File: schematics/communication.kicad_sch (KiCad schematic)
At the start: 9 parts, among them J2 Conn_01x05_Pin, U3 SHT31-DIS

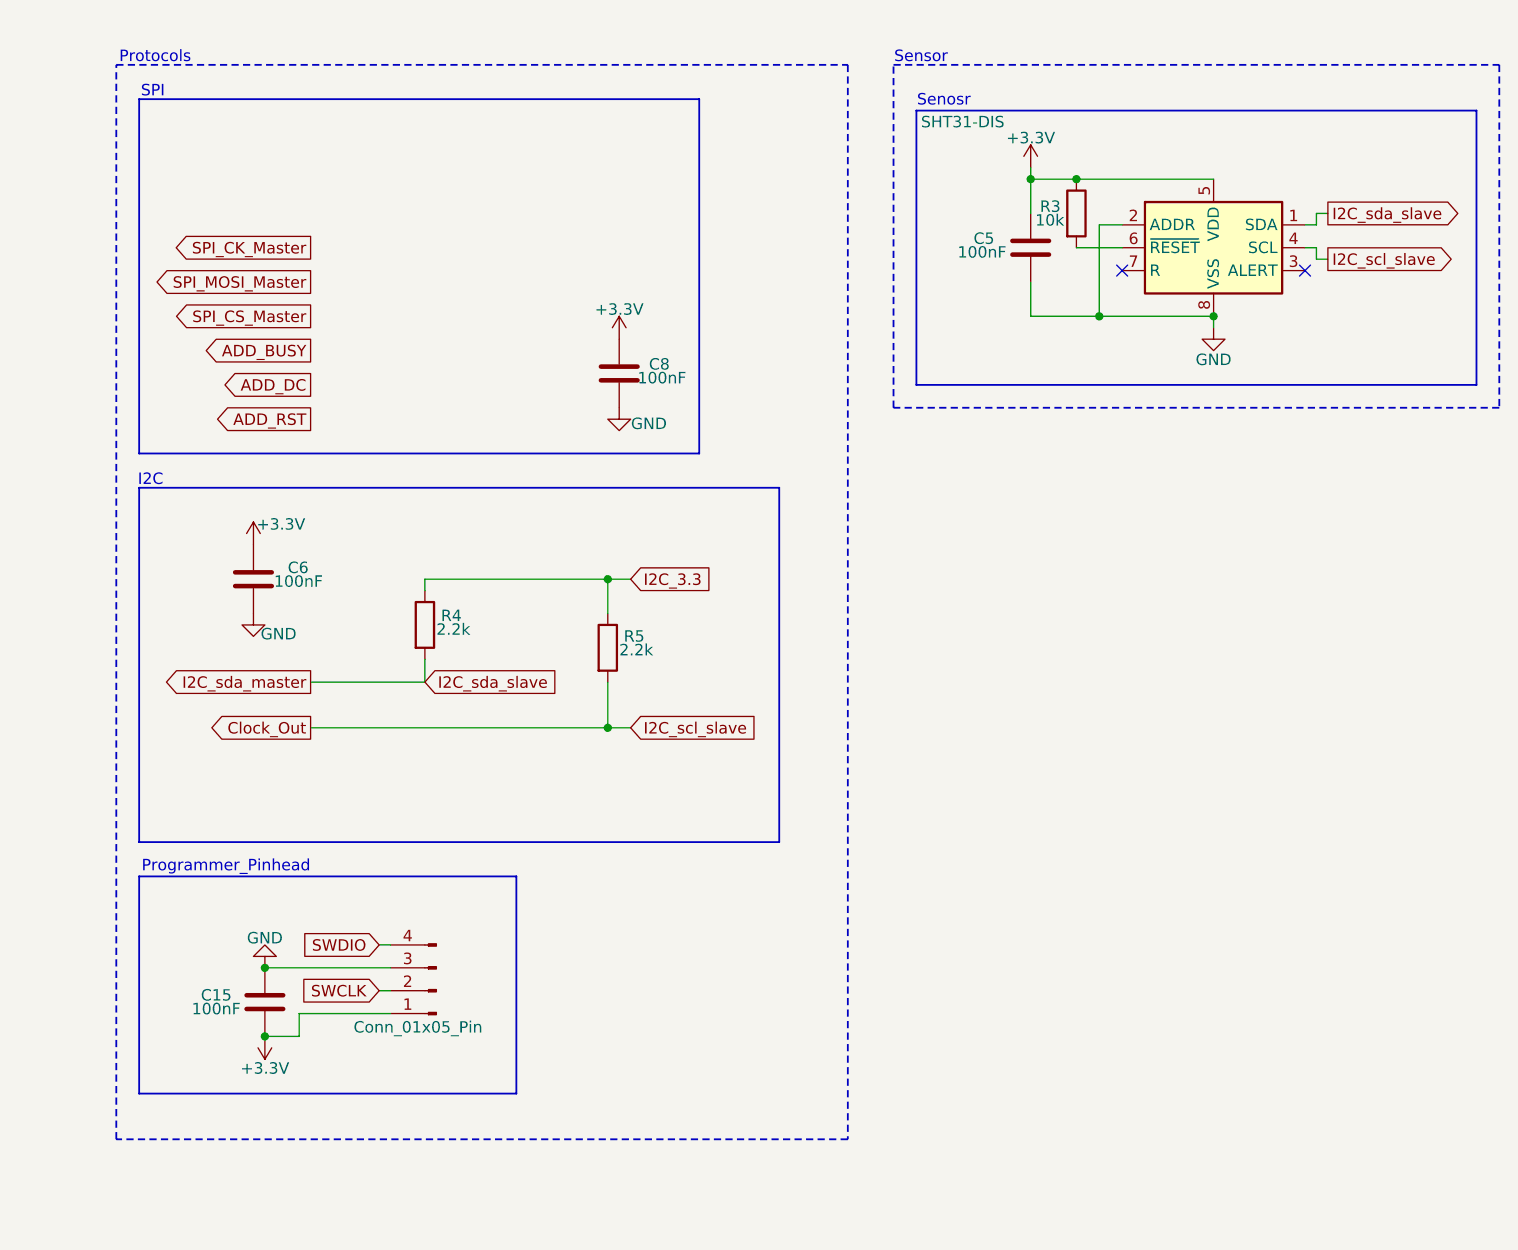
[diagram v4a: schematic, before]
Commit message: 2026-03-01 | 2
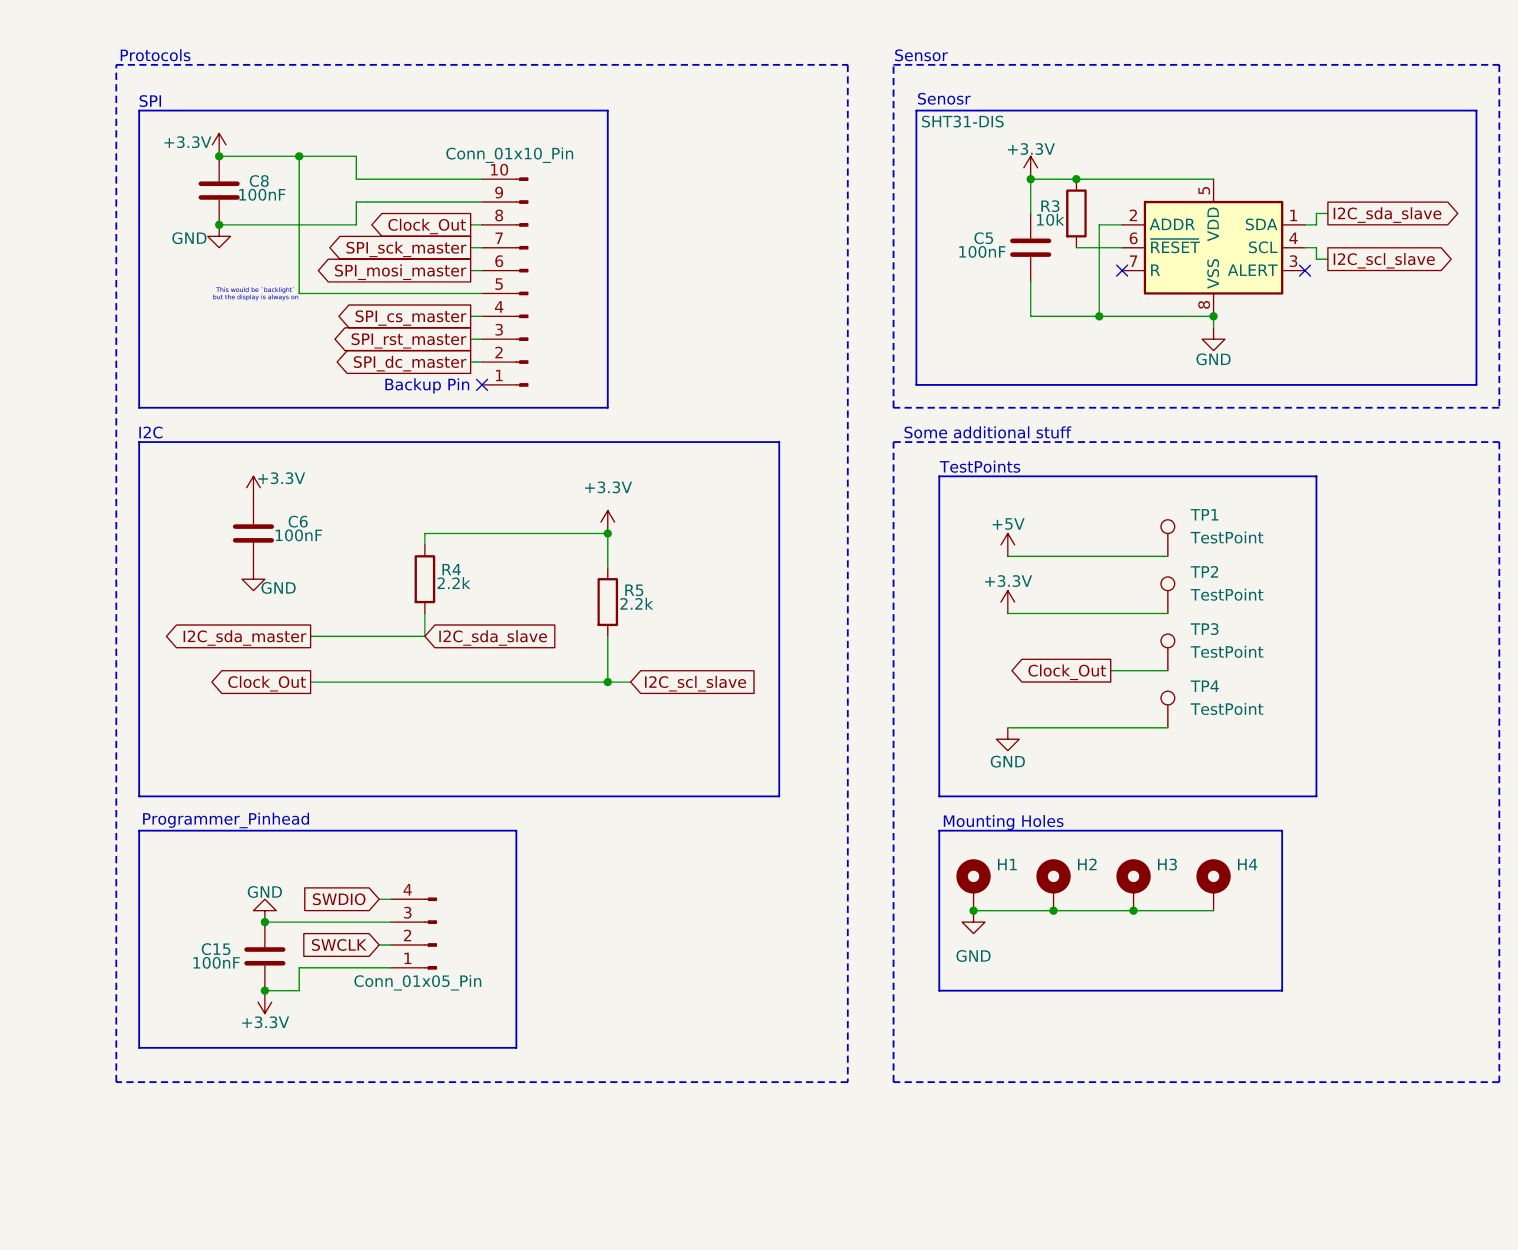
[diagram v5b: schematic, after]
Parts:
- added H1, H2, H3, H4: MountingHole_Pad, MountingHole:MountingHole_2.2mm_M2_DIN965_Pad, symbol Mechanical:MountingHole_Pad
- added J3: Conn_01x10_Pin, Connector_PinHeader_1.00mm:PinHeader_1x10_P1.00mm_Vertical, symbol Connector:Conn_01x10_Pin
- added TP1, TP2, TP3, TP4: TestPoint, TestPoint:TestPoint_Pad_1.0x1.0mm, symbol Connector:TestPoint
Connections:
- net I2C_3.3 is gone; now on net +3.3V: R4.1, R5.1
- net +3.3V: now also J3.10 (Pin_10), J3.5 (Pin_5), TP2.1
- net Clock_Out: now also J3.8 (Pin_8), TP3.1
- net GND: now also H1.1, H2.1, H3.1, H4.1, J3.9 (Pin_9), TP4.1
- new net +5V: TP1.1
- new net SPI_cs_master: J3.4 (Pin_4)
- new net SPI_dc_master: J3.2 (Pin_2)
- new net SPI_mosi_master: J3.6 (Pin_6)
- new net SPI_rst_master: J3.3 (Pin_3)
- new net SPI_sck_master: J3.7 (Pin_7)
- no-connect marks 2 -> 3
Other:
- note added: "Backup Pin"
- note added: "Mounting Holes"
- note added: "Some additional stuff"
- note added: "TestPoints"
- note added: "This would be `backlight` but the display is always on"
- moved on the sheet: C15, C6, C8, R4, R5

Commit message: 2026-03-09 | So-Mo
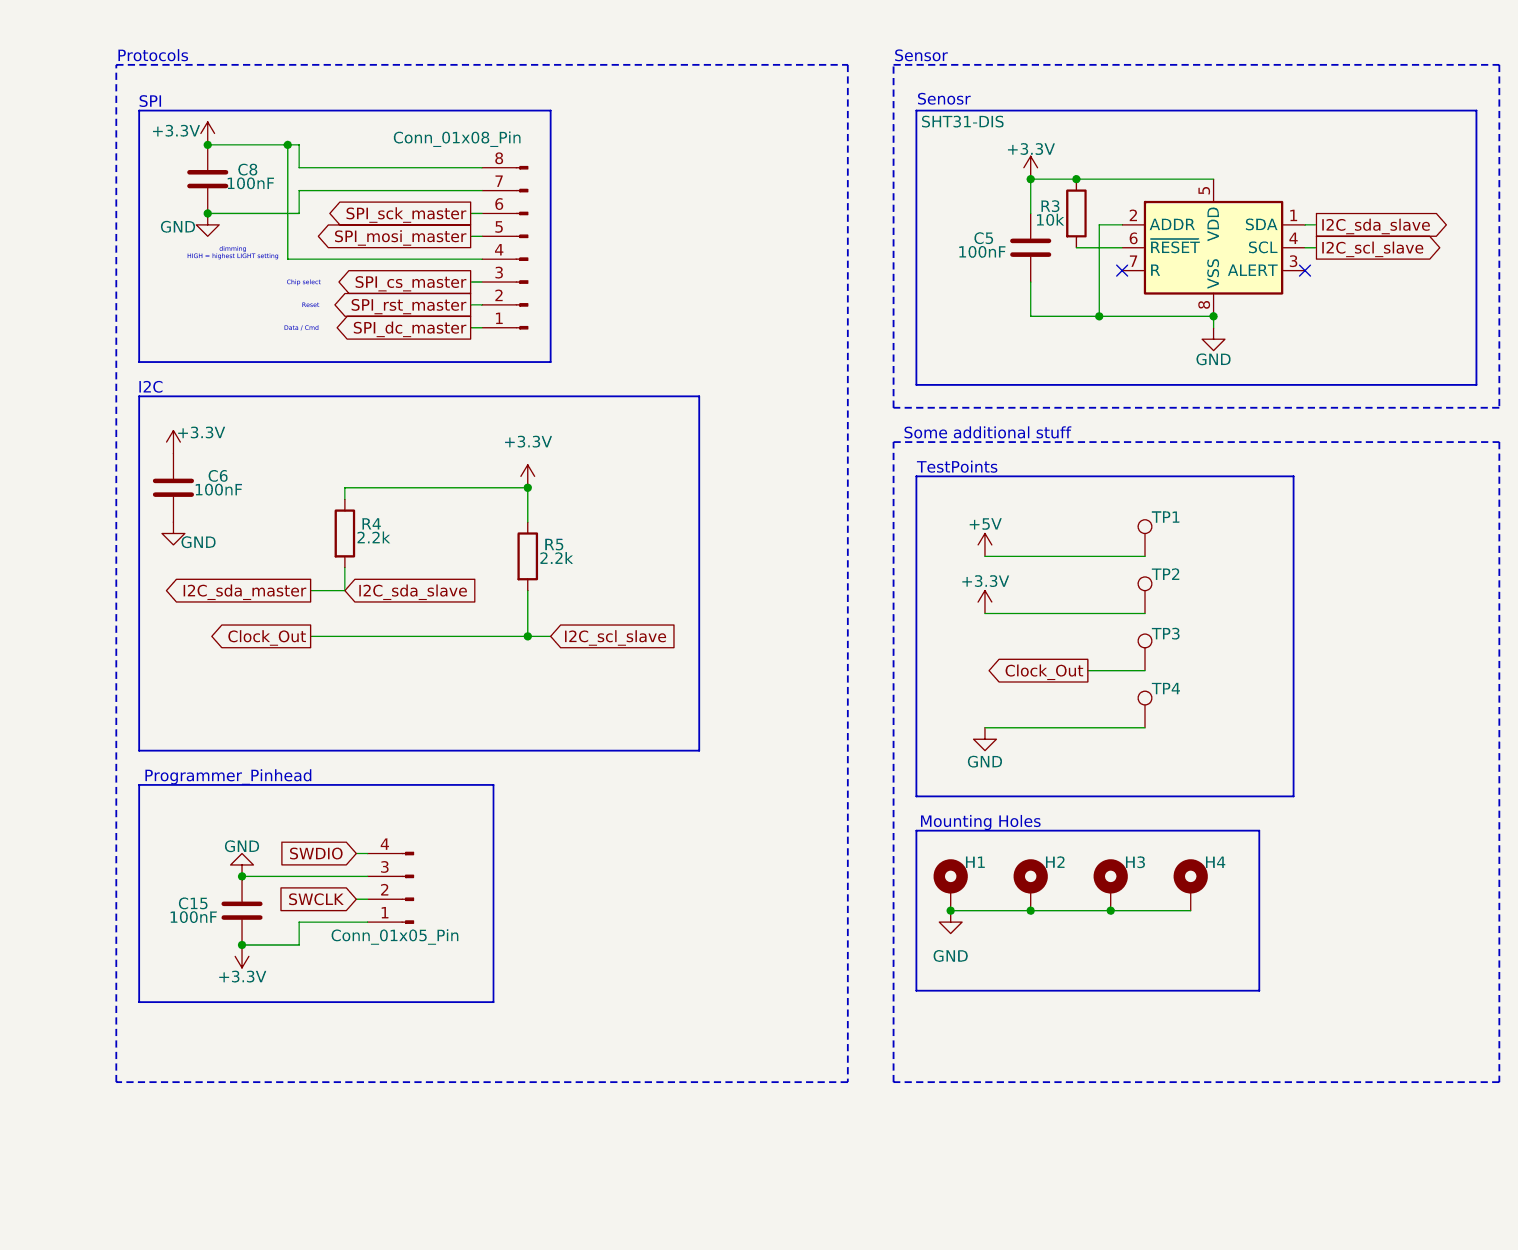
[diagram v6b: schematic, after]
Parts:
- removed J3: Conn_01x10_Pin, Connector_PinHeader_1.00mm:PinHeader_1x10_P1.00mm_Vertical, symbol Connector:Conn_01x10_Pin
- added J4: Conn_01x08_Pin, Connector_PinHeader_1.00mm:PinHeader_1x08_P1.00mm_Vertical, symbol Connector:Conn_01x08_Pin
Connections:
- net +3.3V: now also J4.4 (Pin_4), J4.8 (Pin_8)
- net GND: now also J4.7 (Pin_7)
- net SPI_cs_master: now also J4.3 (Pin_3)
- net SPI_dc_master: now also J4.1 (Pin_1)
- net SPI_mosi_master: now also J4.5 (Pin_5)
- net SPI_rst_master: now also J4.2 (Pin_2)
- net SPI_sck_master: now also J4.6 (Pin_6)
- no-connect marks 3 -> 2
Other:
- note added: "Chip select"
- note added: "Data / Cmd"
- note added: "Reset"
- note added: "dimming HIGH = highest LIGHT setting"
- note removed: "Backup Pin"
- note removed: "This would be `backlight` but the display is always on"
- moved on the sheet: C15, C6, C8, H1, H2, H3, H4, R4, R5, TP1, TP2, TP3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

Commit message: 2026-03-11
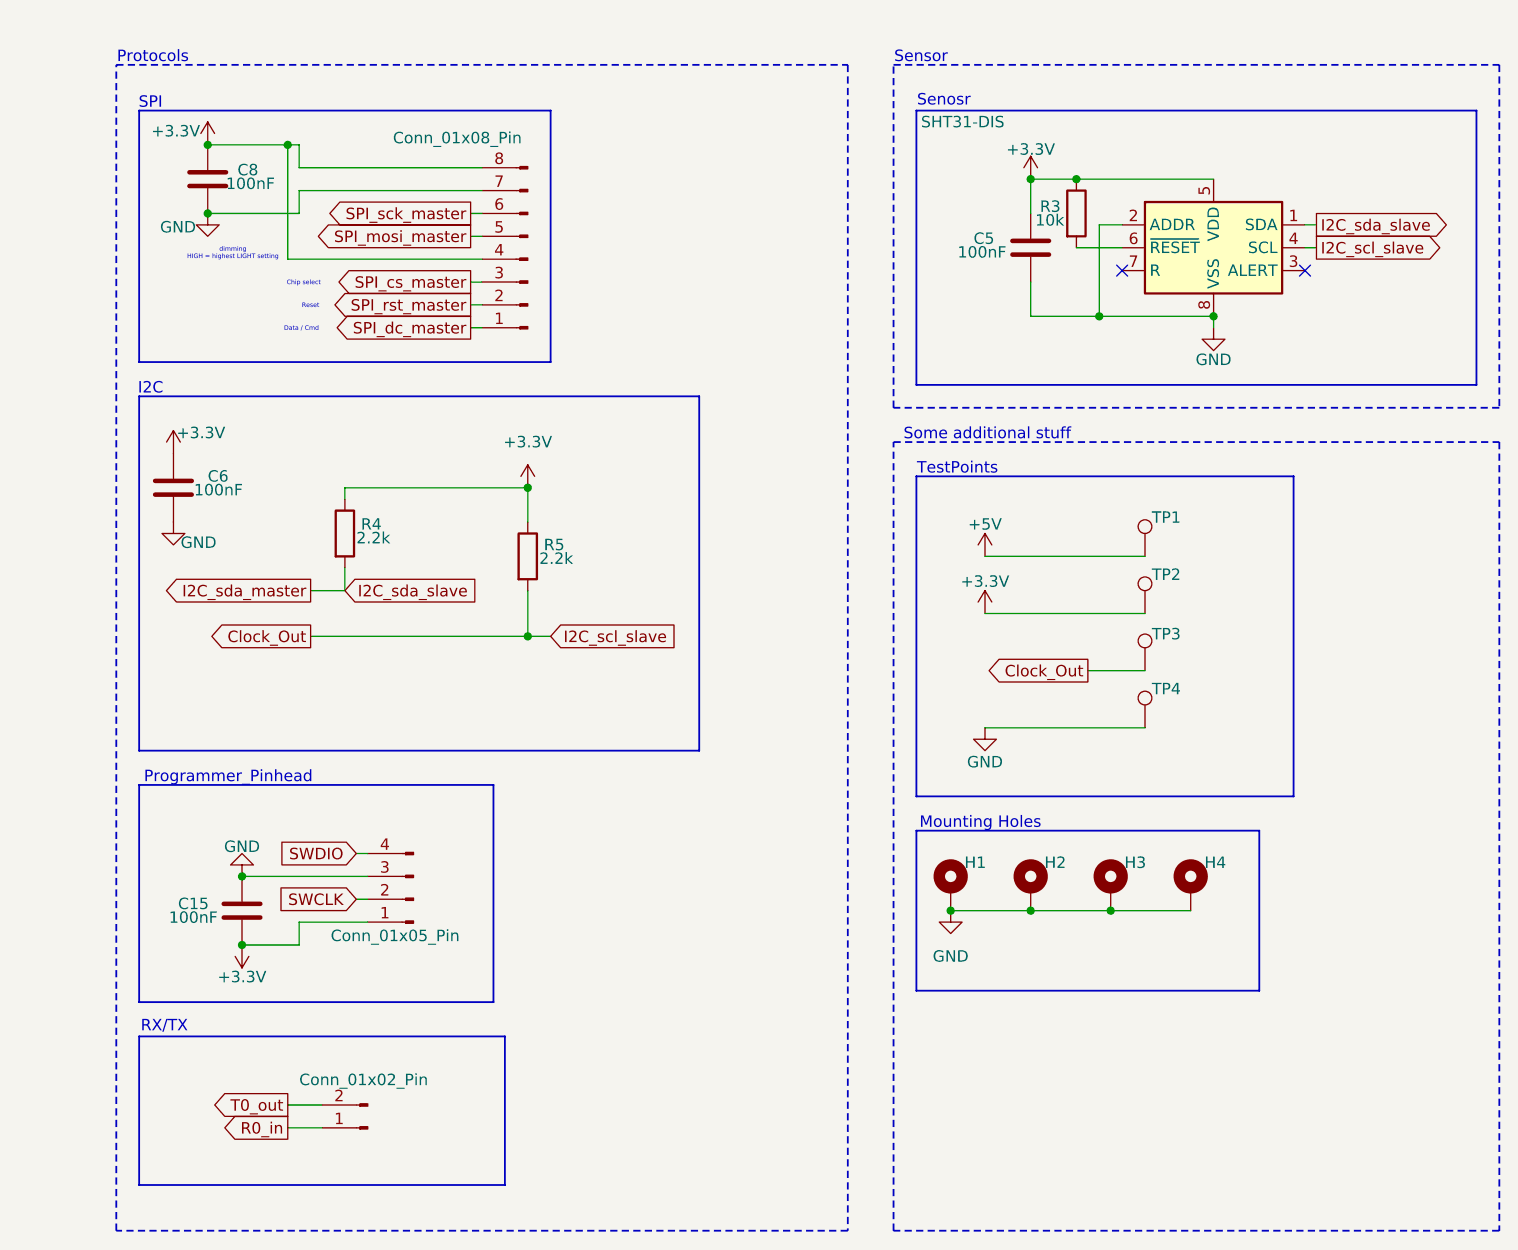
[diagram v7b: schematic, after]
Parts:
- added J3: Conn_01x02_Pin, Connector_PinHeader_2.54mm:PinHeader_1x02_P2.54mm_Vertical, symbol Connector:Conn_01x02_Pin
- J2: footprint Connector_PinHeader_1.00mm:PinHeader_1x04_P1.00mm_Vertical -> Connector_PinHeader_2.54mm:PinHeader_1x05_P2.54mm_Vertical
- J4: footprint Connector_PinHeader_1.00mm:PinHeader_1x08_P1.00mm_Vertical -> Connector_PinHeader_2.54mm:PinHeader_1x08_P2.54mm_Vertical
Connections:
- new net R0_in: J3.1 (Pin_1)
- new net T0_out: J3.2 (Pin_2)
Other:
- note added: "RX/TX"
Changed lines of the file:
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@@
 	(rectangle
 		(start 22.86 21.59)
-		(end 104.14 134.62)
+		(end 104.14 151.13)
 		(stroke
 			(width 0.2)
@@
 	)
 	(rectangle
-		(start 111.76 67.31)
-		(end 153.67 102.87)
+		(start 25.4 129.54)
+		(end 66.04 146.05)
 		(stroke
 			(width 0.2)
@@
 	)
 	(rectangle
-		(start 25.4 58.42)
-		(end 87.63 97.79)
+		(start 111.76 67.31)
+		(end 153.67 102.87)
 		(stroke
 			(width 0.2)
@@
 	)
 	(rectangle
-		(start 25.4 101.6)
-		(end 64.77 125.73)
+		(start 25.4 58.42)
+		(end 87.63 97.79)
 		(stroke
 			(width 0.2)
@@
 	)
 	(rectangle
+		(start 25.4 101.6)
+		(end 64.77 125.73)
+		(stroke
+			(width 0.2)
+			(type default)
+			(color 0 0 0 1)
+		)
+		(fill
+			(type color)
+			(color 255 255 194 1)
+		)
+	)
+	(rectangle
 		(start 109.22 21.59)
 		(end 176.53 59.69)
@@
 	(rectangle
 		(start 109.22 63.5)
-		(end 176.53 134.62)
+		(end 176.53 151.13)
 		(stroke
 			(width 0.2)
@@
 		(exclude_from_sim no)
 		(at 118.872 105.918 0)
+		(effects
+			(font
+				(size 1.27 1.27)
+			)
+		)
+	)
+	(text "RX/TX"
+		(exclude_from_sim no)
+		(at 28.194 128.524 0)
 		(effects
 			(font
@@
 	(wire
 		(pts
+			(xy 45.72 137.16) (xy 41.91 137.16)
+		)
+		(stroke
+			(width 0)
+			(type default)
+		)
+	)
+	(wire
+		(pts
 			(xy 115.57 115.57) (xy 124.46 115.57)
 		)
@@
 	(wire
 		(pts
+			(xy 41.91 139.7) (xy 45.72 139.7)
+		)
+		(stroke
+			(width 0)
+			(type default)
+		)
+	)
+	(wire
+		(pts
 			(xy 36.83 119.38) (xy 43.18 119.38)
 		)
@@
 			(width 0)
 			(type default)
+		)
+	)
+	(global_label "R0_in"
+		(shape output)
+		(at 41.91 139.7 180)
+		(fields_autoplaced yes)
+		(effects
+			(font
+				(size 1.27 1.27)
+			)
+			(justify right)
+		)
+		(property "Intersheetrefs" "${INTERSHEET_REFS}"
+			(at 33.7239 139.7 0)
+			(effects
+				(font
+					(size 1.27 1.27)
+				)
+				(justify right)
+				(hide yes)
+			)
 		)
 	)
@@
 		)
 	)
+	(global_label "T0_out"
+		(shape output)
+		(at 41.91 137.16 180)
+		(fields_autoplaced yes)
+		(effects
+			(font
+				(size 1.27 1.27)
+			)
+			(justify right)
+		)
+		(property "Intersheetrefs" "${INTERSHEET_REFS}"
+			(at 32.7564 137.16 0)
+			(effects
+				(font
+					(size 1.27 1.27)
+				)
+				(justify right)
+				(hide yes)
+			)
+		)
+	)
 	(global_label "I2C_sda_slave"
 		(shape output)
@@
 				(justify right)
 				(hide yes)
+			)
+		)
+	)
+	(symbol
+		(lib_id "Connector:Conn_01x02_Pin")
+		(at 50.8 139.7 180)
+		(unit 1)
+		(exclude_from_sim no)
+		(in_bom yes)
+		(on_board yes)
+		(dnp no)
+		(property "Reference" "J3"
+			(at 52.07 137.1599 0)
+			(effects
+				(font
+					(size 1.27 1.27)
+				)
+				(justify right)
+				(hide yes)
+			)
+		)
+		(property "Value" "Conn_01x02_Pin"
+			(at 43.18 134.366 0)
+			(effects
+				(font
+					(size 1.27 1.27)
+				)
+				(justify right)
+			)
+		)
+		(property "Footprint" "Connector_PinHeader_2.54mm:PinHeader_1x02_P2.54mm_Vertical"
+			(at 50.8 139.7 0)
+			(effects
+				(font
+					(size 1.27 1.27)
+				)
+				(hide yes)
+			)
+		)
+		(property "Datasheet" "~"
+			(at 50.8 139.7 0)
+			(effects
+				(font
+					(size 1.27 1.27)
+				)
+				(hide yes)
+			)
+		)
+		(property "Description" "Generic connector, single row, 01x02, script generated"
+			(at 50.8 139.7 0)
+			(effects
+				(font
+					(size 1.27 1.27)
+				)
+				(hide yes)
+			)
+		)
+		(property "Sim.Library" ".\\"
+			(at 50.8 139.7 0)
+			(effects
+				(font
+					(size 1.27 1.27)
+				)
+				(hide yes)
+			)
+		)
+		(pin "2"
+		)
+		(pin "1"
+		)
+		(instances
+			(project ""
+				(path "/c936f4ed-9370-4c35-ba8e-26b0afd3f3bd/83b5ba43-ad0f-481c-b93f-0dd69f5fe66c"
+					(reference "J3")
+					(unit 1)
+				)
 			)
 		)
@@
 			)
 		)
-		(property "Footprint" "Connector_PinHeader_1.00mm:PinHeader_1x04_P1.00mm_Vertical"
+		(property "Footprint" "Connector_PinHeader_2.54mm:PinHeader_1x05_P2.54mm_Vertical"
 			(at 55.88 114.3 0)
 			(effects
@@
 			)
 		)
-		(property "Footprint" "Connector_PinHeader_1.00mm:PinHeader_1x08_P1.00mm_Vertical"
+		(property "Footprint" "Connector_PinHeader_2.54mm:PinHeader_1x08_P2.54mm_Vertical"
 			(at 68.58 43.18 0)
 			(effects
